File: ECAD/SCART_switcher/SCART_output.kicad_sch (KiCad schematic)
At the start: 7 parts, among them J2 RCA Left, J3 RCA Right, J4 SCART-F, Q3 BC847

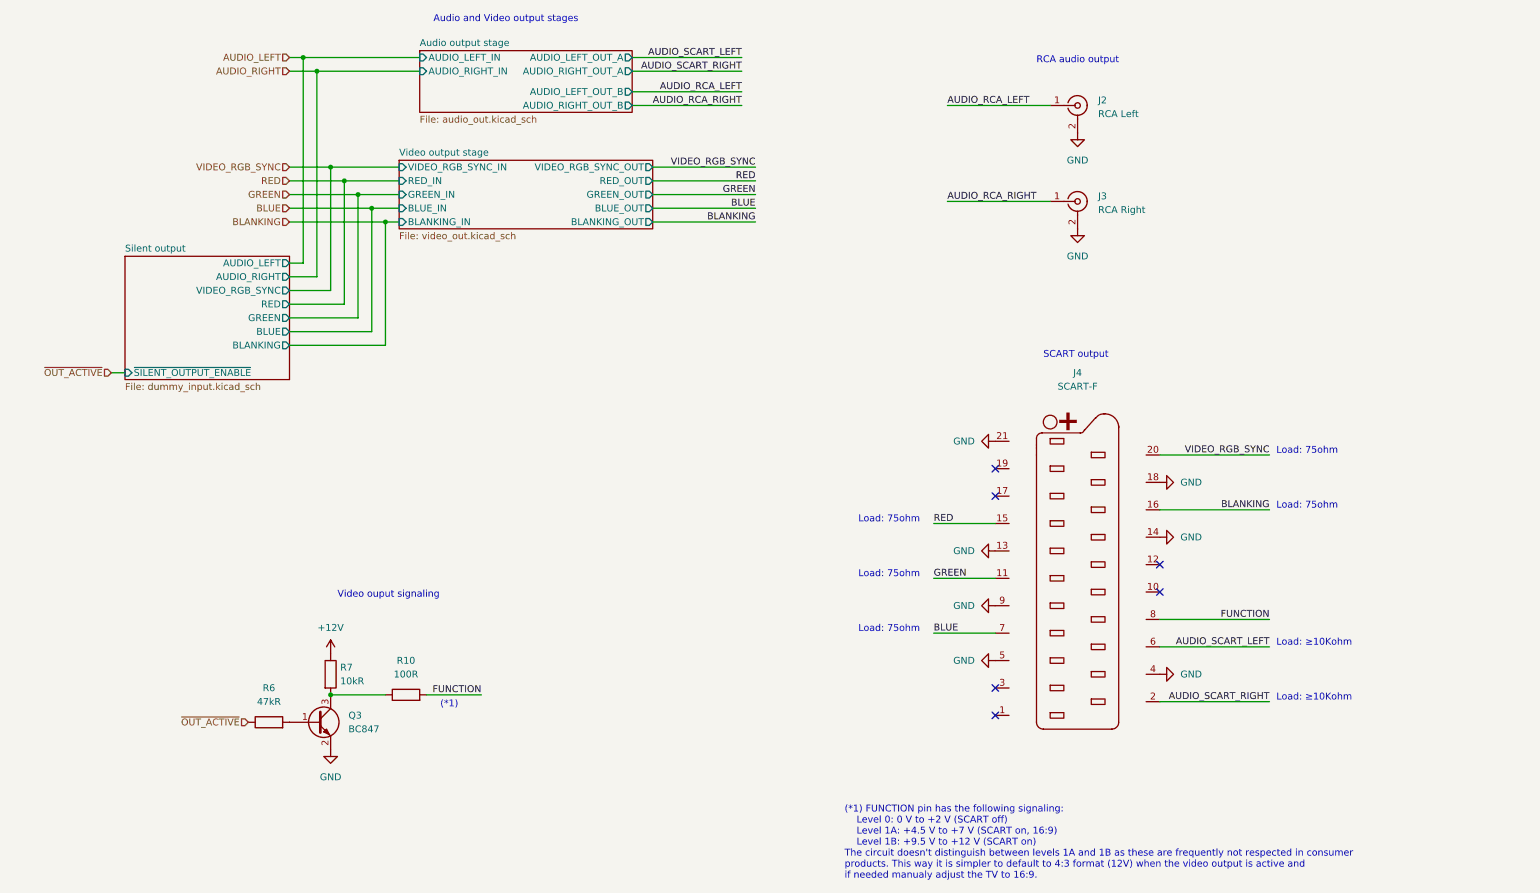
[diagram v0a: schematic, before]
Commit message: Progressed ECAD
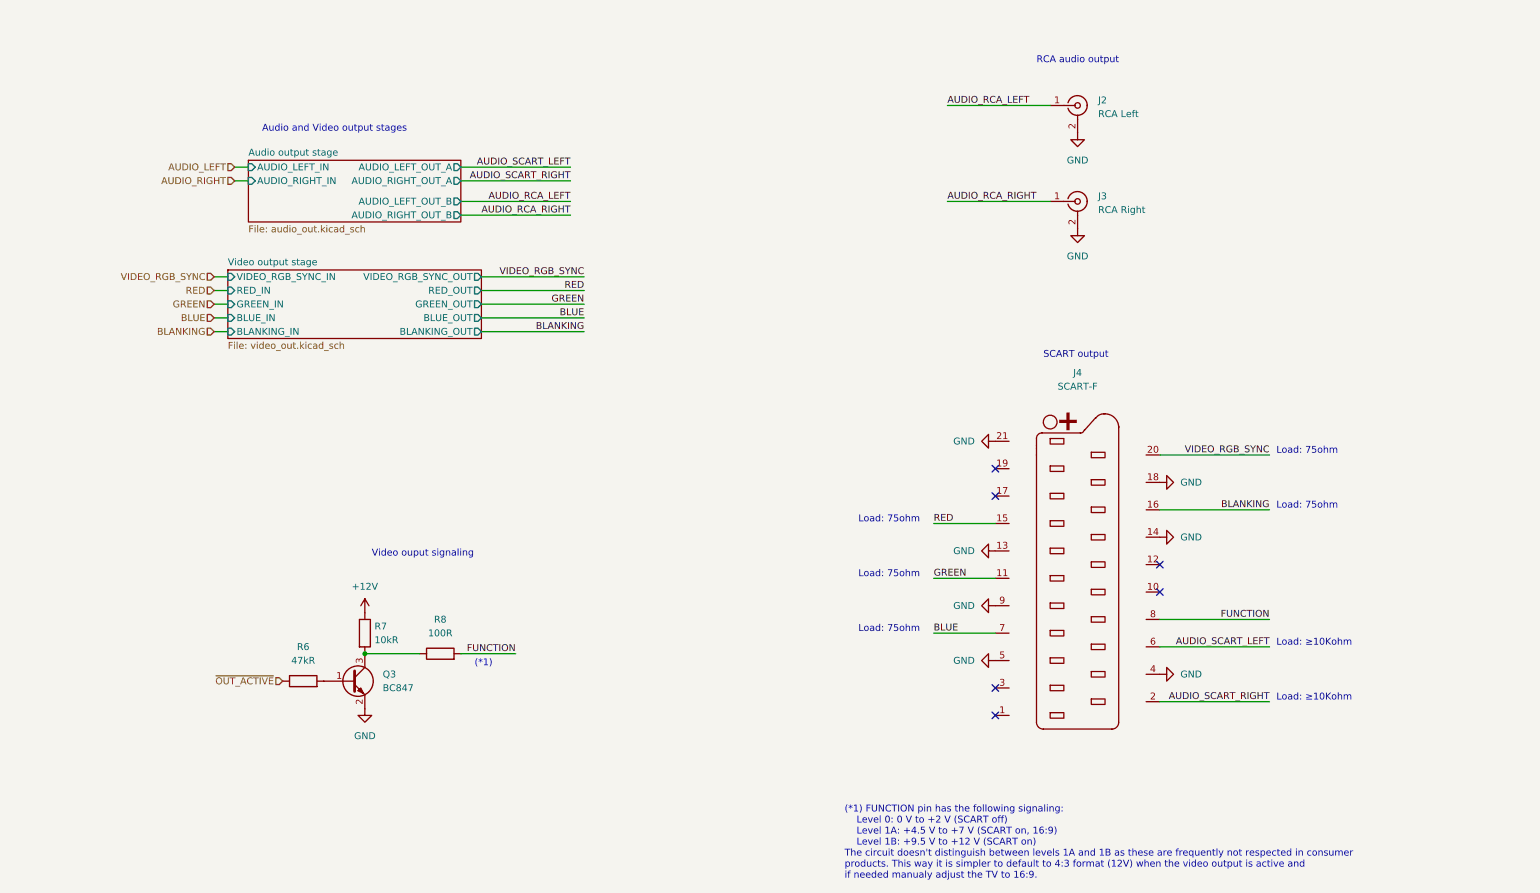
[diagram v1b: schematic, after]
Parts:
- renumbered R10 to R8
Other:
- removed sheet Silent output
- moved on the sheet: Q3, R6, R7, R8
